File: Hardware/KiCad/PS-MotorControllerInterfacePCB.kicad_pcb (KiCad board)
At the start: 2 copper layers, 59.1 x 75.7 mm, 118 parts, among them IC1 LM74502HDDFR, IC2 LM74502HDDFR, J1 CAN board out, J2 PWR board, J3 CAN board in, J4 53307-2471, J5 PWR Moco, J6 Candapter, J7 CAN board -> mppt +moco, J8 CAN mppts + moco -> board, J9 Conn_01x06, Q1 IRLML0030, Q2 IRLML0030, Q3 NVMFWS1D7N04XMT1G, Q4 NVMFWS1D7N04XMT1G, Q5 771-BUK6M61-60PX, Q6 NVMFWS1D7N04XMT1G, Q7 NVMFWS1D7N04XMT1G, U1 LMR33630ADDA

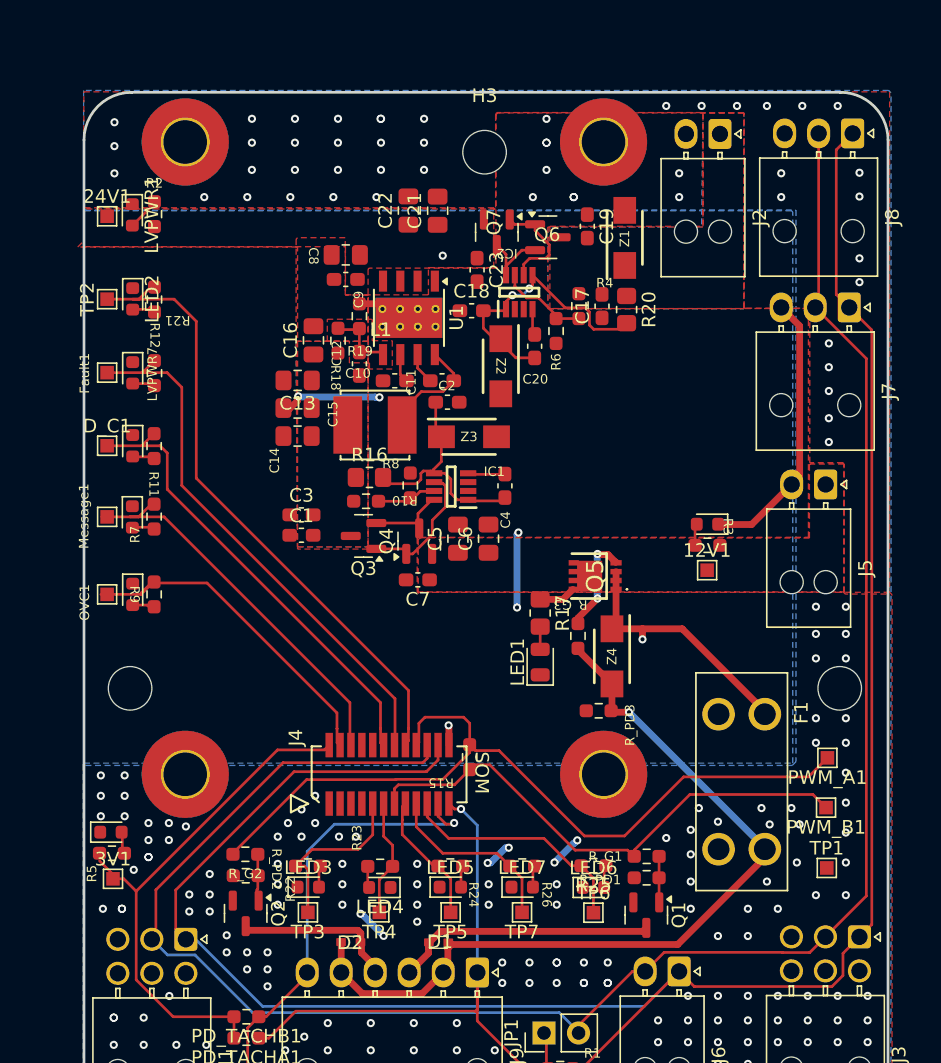
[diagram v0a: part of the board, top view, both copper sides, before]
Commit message: sch changes, pre pcb changes
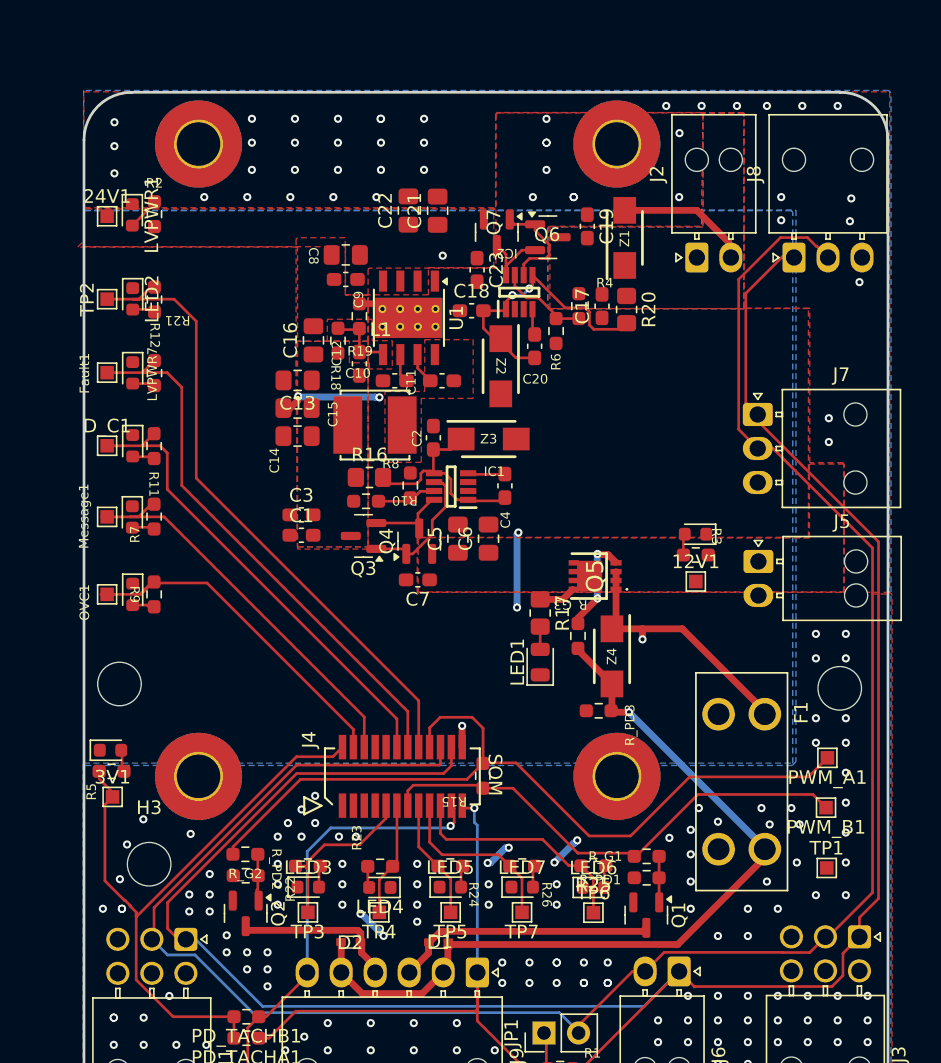
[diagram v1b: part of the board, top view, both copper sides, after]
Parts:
- J1, J3: footprint Connector_Molex:Molex_Nano-Fit_105314-xx06_2x03_P2.50mm_Horizontal -> UTSVT_Connectors:105314-1306
- J2, J5, J6: footprint Connector_Molex:Molex_Nano-Fit_105313-xx02_1x02_P2.50mm_Horizontal -> UTSVT_Connectors:105313-2102
- J7, J8: footprint Connector_Molex:Molex_Nano-Fit_105313-xx03_1x03_P2.50mm_Horizontal -> UTSVT_Connectors:105313-1103
- J9: footprint Connector_Molex:Molex_Nano-Fit_105313-xx06_1x06_P2.50mm_Horizontal -> UTSVT_Connectors:105313-1106
- moved H3 57.8 mm to (157.8, 92.5)
- moved J7 10.3 mm to (202.5, 59.5), turned to 0 degrees
- moved J8 10.1 mm to (205.2, 47.9), turned to 90 degrees
- moved J2 9.24 mm to (198.1, 47.9), turned to 90 degrees
- moved J5 7.51 mm to (202.6, 70.3), turned to 0 degrees
- moved 3V1 6.02 mm to (155.1, 87.6)
- moved LVPWR3 6.02 mm to (155.0, 84.2)
- moved R5 6.02 mm to (155.0, 85.7)
- moved C2 2.81 mm to (178.7, 61.2), turned to -90 degrees
- moved R15 1.68 mm to (182.3, 86.0)
- moved Z3 1.46 mm to (182.8, 61.3)
- moved 12V1 1.18 mm to (198.0, 71.8)
- moved LVPWR2 1.15 mm to (197.9, 68.3)
- moved R3 1.11 mm to (198.0, 69.8)
- moved J4 0.99 mm to (176.4, 86.1)
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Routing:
- net GND: track 44.5 -> 33.8 mm, vias 234 -> 219
- net Net-(U1-SW): track 8.25 -> 0.00 mm
- net +3V3: track 38.4 -> 46.3 mm
- net /CAN_H: track 155.6 -> 152.9 mm
- net /PWM_FAN_B: track 38.9 -> 36.4 mm
- net /RPP_EN12: track 17.3 -> 15.6 mm
- net /CAN_L: track 146.3 -> 147.8 mm
- net /FAN_B_TACHO: track 34.7 -> 33.6 mm
- net /LED3: track 9.74 -> 8.82 mm
- net /MESSAGE: track 28.9 -> 29.5 mm
- net /D_C: track 34.3 -> 34.9 mm
- net /S_OC: track 25.5 -> 26.1 mm
- net /M_FAULT: track 40.3 -> 40.8 mm
- added copper zone on F.Cu, net Net-(U1-SW)
